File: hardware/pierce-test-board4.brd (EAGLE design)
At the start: 25.4 x 25.4 mm, 8 parts

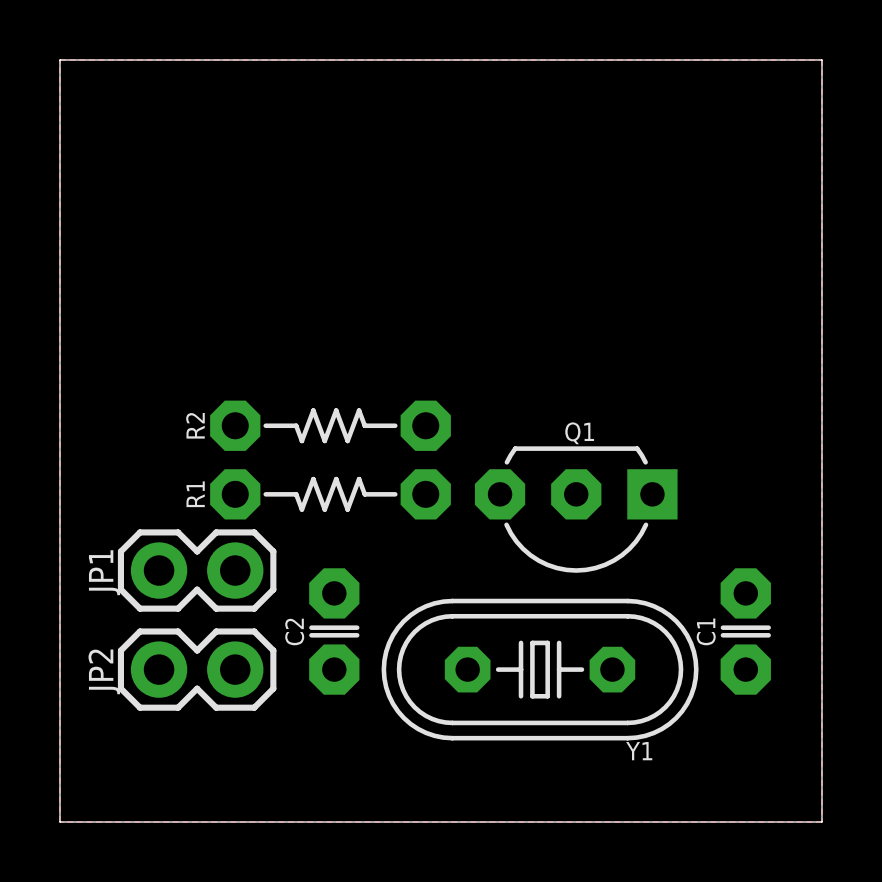
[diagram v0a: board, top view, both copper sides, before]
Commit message: yet another test pcb
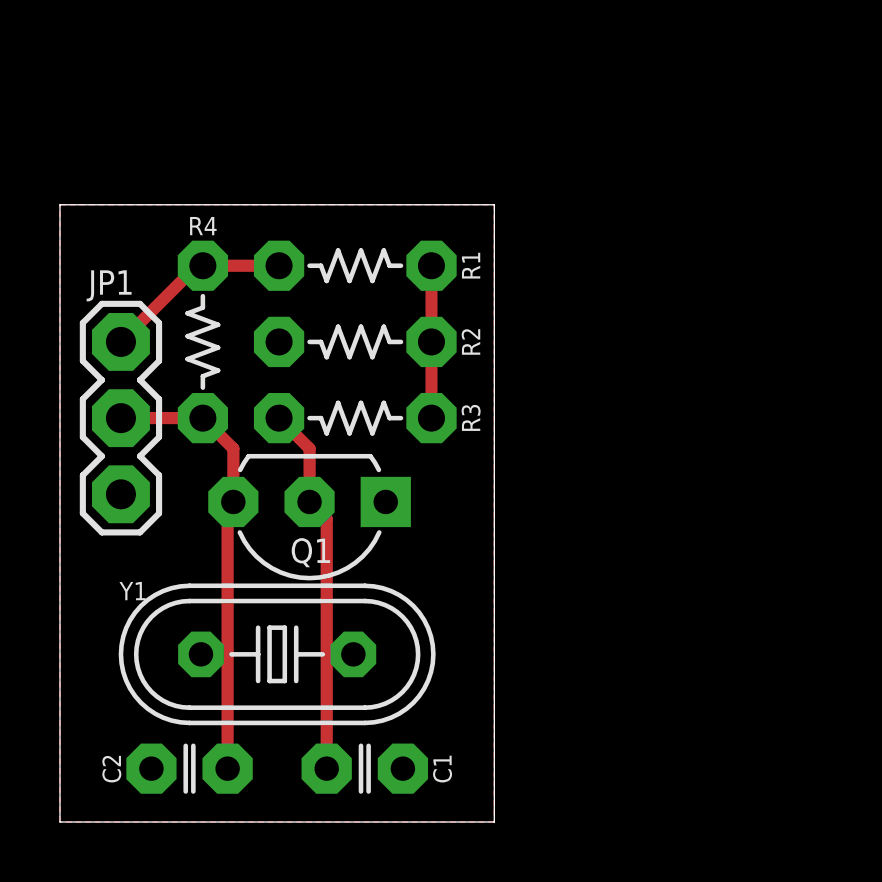
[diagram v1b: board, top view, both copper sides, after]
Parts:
- removed JP2: M02PTH, A_butts:1X02
- added R3: 39k, A_butts:RESISTOR-AXIAL-PTH-5.08MM
- added R4: 1.2k, A_butts:RESISTOR-AXIAL-PTH-5.08MM
- added U$1: (no value), A_butts:CC-BY-SA-4.0-NO-URL
- C1: value (none) -> 100pF
- C2: value (none) -> 27pF
- JP1: value M02PTH -> (none); device A_butts:1X02 -> A_butts:1X03
- Q1: value (none) -> 1N3904
- R1: value (none) -> 4.7k
- R2: value (none) -> 1.5k
- Y1: value (none) -> $foo
- moved C1 13.5 mm to (10.2, 1.78), turned to 0 degrees
- moved Q1 8.89 mm to (8.32, 10.7)
- moved Y1 8.78 mm to (7.24, 5.59)
- moved R1 7.66 mm to (9.84, 18.5)
- moved C2 6.65 mm to (4.32, 1.78), turned to 180 degrees
- moved R2 2.91 mm to (9.84, 16.0)
- moved JP1 2.84 mm to (2.03, 10.9), turned to 90 degrees
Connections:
- removed net N$1: C2.1, Y1.2
- new net N$2: R1.P$1, R2.P$2, R3.P$1
- net GND: now also Q1.1, R2.P$1; no longer JP2.1
- net N$4: now also Q1.2, R3.P$2
- net VCC: now also JP1.3, R4.P$1; no longer JP1.2
- net XOUT: now also C2.1, JP1.2, Q1.3, R4.P$2, Y1.2; no longer JP2.2
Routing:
- net XOUT: track 0.00 -> 15.8 mm
- net N$4: track 0.00 -> 13.2 mm
- net VCC: track 0.00 -> 6.32 mm
- net N$2: track 0.00 -> 5.08 mm
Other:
- board size 25.4 x 25.4 mm -> 14.5 x 20.6 mm
